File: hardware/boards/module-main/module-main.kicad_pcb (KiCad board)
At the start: 4 copper layers, 48.5 x 108.5 mm, 177 parts, among them J1 2x8 2.54mm shrouded box heade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, J2 2x10 2.54mm pin header, J3 Neutrik NE8FAV, J4 JST B2B-XH-A, Q1 PSMN2R0-30YLE, SW1 NKK M2011SD4G01, U1 LT3042EMSE, U10 OPA2197, U11 OPA2197, U12 OPA2197, U13 ADP7118AUJZ-5.0, U14 RPA20-2412SAW, U15 74AHCT14, U2 LT1641-1IS8, U3 DAC8568ICPW, U4 74AHCT125, U5 OPA2197, U6 INA828IDR, U7 OPA2197, U8 OPA2197IDR, U9 OPA2197

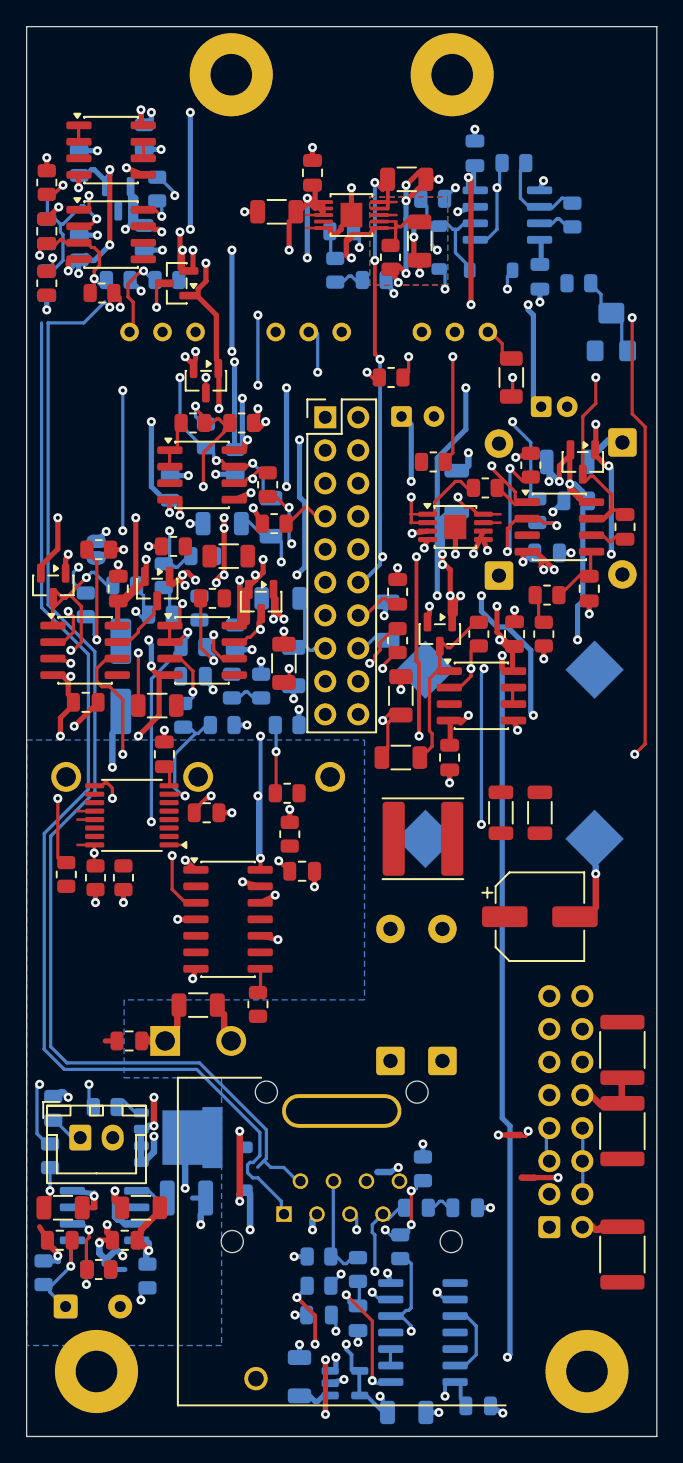
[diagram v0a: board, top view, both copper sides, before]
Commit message: module-main: routing state, 31 connections left after Freerouting the remainder on three layers
Co-Authored-By: Claude Opus 5.5 <noreply@anthropic.com>
Claude-Session: https://claude.ai/code/session_01LmB4muFXnoLprWX4JzuJ5A
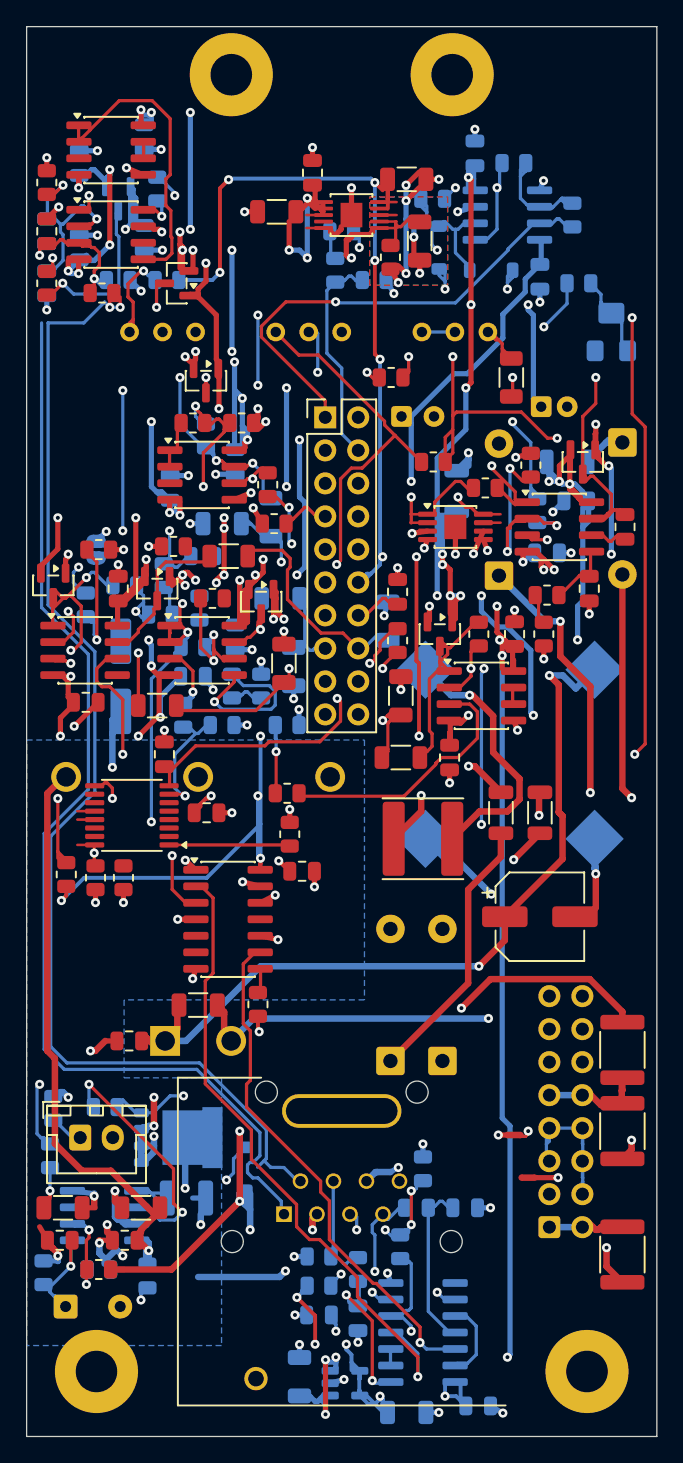
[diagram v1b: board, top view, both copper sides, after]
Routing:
- net /DAC_AVDD: track 84.7 -> 146.9 mm, vias 11 -> 15
- net /power-entry/ISO_VIN_POS: track 1.57 -> 62.4 mm, vias 0 -> 2
- net /power-entry/NEG12_PTC3: track 0.00 -> 59.0 mm, vias 0 -> 3
- net /VREFOUT: track 1.00 -> 56.6 mm, vias 0 -> 2
- net MODULE_ANALOG_POS12: track 293.6 -> 347.9 mm
- net /digital-and-supervision/SCLK_BUF: track 0.00 -> 50.6 mm, vias 0 -> 1
- net ISO_POS12: track 9.66 -> 55.5 mm
- net /power-entry/POS12_PTC1: track 0.00 -> 45.6 mm, vias 0 -> 2
- net MODULE_ANALOG_NEG12: track 260.8 -> 302.5 mm, vias 47 -> 48
- net /power-entry/ISO_VIN_NEG: track 4.40 -> 45.8 mm, vias 1 -> 2
- net /digital-and-supervision/CS_BUF: track 0.00 -> 39.7 mm, vias 0 -> 1
- net /BREATH_SHAPED: track 1.33 -> 36.8 mm, vias 0 -> 1
- net /PITCH_JACK: track 4.11 -> 38.2 mm
- net /pitch-stage/VREF_SUM: track 12.3 -> 36.4 mm, vias 2 -> 4
- net /RESP_WIPER: track 0.00 -> 23.8 mm, vias 0 -> 1
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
